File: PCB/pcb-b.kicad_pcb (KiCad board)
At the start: 2 copper layers, 116.9 x 83.4 mm, 104 parts, among them IC2 BDX34C, IC3 BDX34C, K1 RT42xxxx, Q1 D45VH10, Q10 BC337, Q11 BC337, Q12 BC327, Q13 BC337, Q14 D45VH10, Q15 D45VH10, Q16 BC337, Q17 BC337, Q18 BC327, Q19 BC327, Q2 D45VH10, Q20 BC327, Q3 BC337, Q4 BC337, Q5 BC337, Q6 BC337, Q7 BC337, Q8 BC337, Q9 BC337, U1 L7805, U2 L7805, U3 L7805, U4 ATmega16L-8P

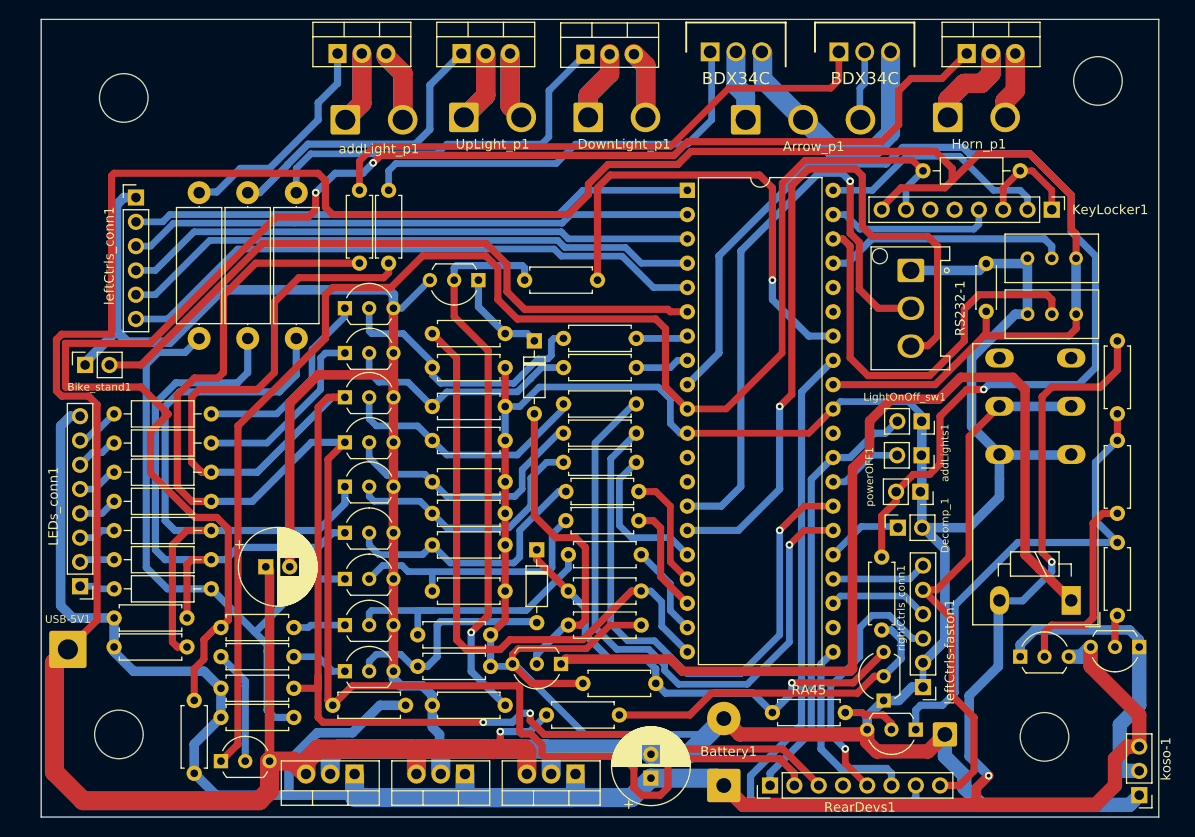
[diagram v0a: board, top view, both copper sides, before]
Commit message: fixes
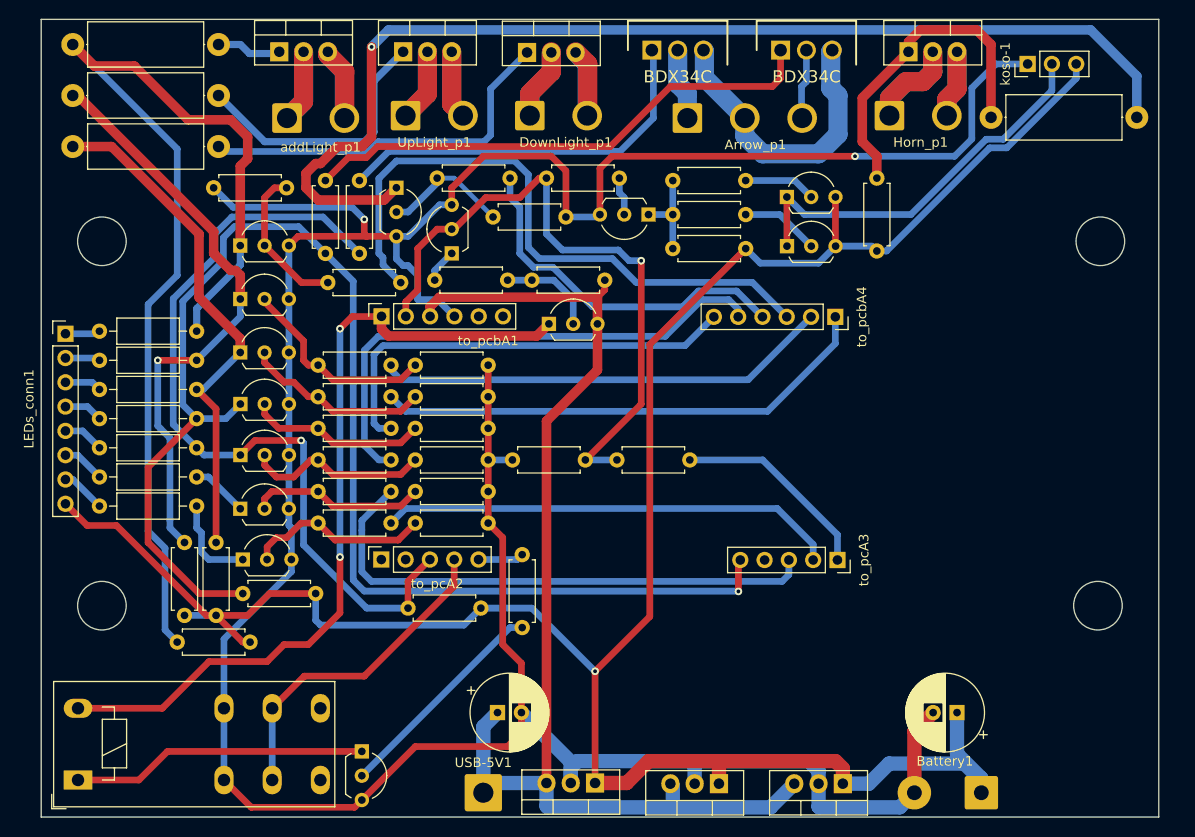
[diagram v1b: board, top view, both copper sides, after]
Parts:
- removed Bike_stand1, Decomp_1, LightOnOff_sw1, addLights1, powerOFF1: Conn_01x02, Connector_PinSocket_2.54mm:PinSocket_1x02_P2.54mm_Vertical
- removed C2: 100nF, Capacitor_THT:C_Disc_D4.3mm_W1.9mm_P5.00mm
- removed D3, D4: 2V, Diode_THT:D_DO-35_SOD27_P7.62mm_Horizontal
- removed KeyLocker1, RearDevs1: Conn_01x08, Connector_PinHeader_2.54mm:PinHeader_1x08_P2.54mm_Vertical
- removed Q19, Q20: BC327, Package_TO_SOT_THT:TO-92L_Inline_Wide
- removed R1: 1K, Resistor_THT:R_Axial_DIN0207_L6.3mm_D2.5mm_P10.16mm_Horizontal
- removed RA45: 10K, Resistor_THT:R_Axial_DIN0207_L6.3mm_D2.5mm_P7.62mm_Horizontal
- removed RA46, RA47: 3K, Resistor_THT:R_Axial_DIN0207_L6.3mm_D2.5mm_P7.62mm_Horizontal
- removed RA48, RA49: 100K, Resistor_THT:R_Axial_DIN0207_L6.3mm_D2.5mm_P7.62mm_Horizontal
- removed RS232-1: Conn_01x03, Connector_Hirose:Hirose_DF63M-3P-3.96DSA_1x03_P3.96mm_Vertical
- removed RV1, RV2: 10K, Potentiometer_THT:Potentiometer_Bourns_3296W_Vertical
- removed U4: ATmega16L-8P, Package_DIP:DIP-40_W15.24mm
- removed leftCtrls-faston1: Conn_01x01, Connector_Wire:SolderWire-0.75sqmm_1x01_D1.25mm_OD2.3mm
- removed leftCtrls_conn1, rightCtrls_conn1: Conn_01x06, Connector_PinHeader_2.54mm:PinHeader_1x06_P2.54mm_Vertical
- added to_pcA2: Conn_01x05, Connector_PinSocket_2.54mm:PinSocket_1x05_P2.54mm_Vertical, F.Cu at (135.1, 112.2)
- added to_pcA3: Conn_01x05, Connector_PinSocket_2.54mm:PinSocket_1x05_P2.54mm_Vertical, F.Cu at (182.8, 112.2)
- added to_pcbA1: Conn_01x06, Connector_PinSocket_2.54mm:PinSocket_1x06_P2.54mm_Vertical, F.Cu at (135.2, 86.7)
- added to_pcbA4: Conn_01x06, Connector_PinSocket_2.54mm:PinSocket_1x06_P2.54mm_Vertical, F.Cu at (182.6, 86.8)
- Q12: value BC327 -> BC337
- Q16, Q17: value BC337 -> BC327
- RA15: footprint Resistor_THT:R_Axial_DIN0207_L6.3mm_D2.5mm_P7.62mm_Horizontal -> Resistor_THT:R_Axial_DIN0414_L11.9mm_D4.5mm_P15.24mm_Horizontal
- RA23: value 5K -> 100K
- RA29: value 10K -> 1K
- RA31: value 100K -> 3K
- RA33: value 10K -> 3K
- RA41: value 4K -> 100K
- RA43, RA44: value 100K -> 10K
- RA7: value 1K -> 5K
- RA8: value 4K -> 10K
- moved K1 105.5 mm to (103.4, 135.2), turned to 0 degrees
- moved RA15 103.0 mm to (214.1, 65.9)
- moved RA42 89.9 mm to (187.0, 79.9)
- moved koso-1 77.3 mm to (202.7, 60.3), turned to 90 degrees
- moved RA29 59.3 mm to (140.7, 82.9), turned to 0 degrees
- moved Q12 58.3 mm to (142.5, 80.2), turned to 90 degrees
- moved Q16 57.2 mm to (152.7, 87.5), turned to 0 degrees
- moved Q18 53.6 mm to (177.5, 74.3), turned to 0 degrees
- moved RA7 52.2 mm to (141.0, 72.3), turned to 0 degrees
- moved RA30 51.2 mm to (165.6, 79.6)
- moved Q13 47.9 mm to (163.1, 76.1)
- moved RA31 46.8 mm to (173.2, 76.1), turned to 180 degrees
- moved Q9 46.0 mm to (136.7, 73.3), turned to -90 degrees
- moved USB-5V1 45.9 mm to (145.8, 136.5)
- moved RA34 44.8 mm to (125.2, 73.3), turned to 180 degrees
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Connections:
- K1 pad A2: +12V -> tempPower
- Q11 pad 1: Net-(Q11-Pad1) -> Net-(K1-PadA1)
- Q11 pad 2: Net-(D4-Pad2) -> Net-(Q11-Pad2)
- Q12 pad 1: tempPower -> Net-(Q12-Pad1)
- Q12 pad 2: Net-(Q12-Pad2) -> i_powerOFF
- Q12 pad 3: +5V -> GND
- Q13 pad 1: Net-(K1-PadA1) -> Net-(Q13-Pad1)
- Q13 pad 2: Net-(D3-Pad2) -> Net-(Q13-Pad2)
- Q16 pad 1: Net-(Q16-Pad1) -> tempPower
- Q16 pad 3: GND -> +5V
- Q17 pad 1: Net-(D3-Pad1) -> Net-(Q17-Pad1)
- Q17 pad 3: GND -> +12V
- Q18 pad 1: GND -> Net-(Q17-Pad1)
- Q18 pad 3: Net-(D4-Pad1) -> +12V
- RA23 pad 1: Net-(Q9-Pad2) -> Net-(Q16-Pad2)
- RA23 pad 2: o_horn -> +5V
- RA29 pad 1: Net-(Q18-Pad2) -> Net-(Q12-Pad1)
- RA29 pad 2: i_powerOFF -> Net-(Q16-Pad2)
- RA30 pad 1: Net-(D4-Pad2) -> Net-(Q13-Pad1)
- RA30 pad 2: GND -> +12V
- RA31 pad 1: Net-(D3-Pad2) -> Net-(Q17-Pad2)
- RA31 pad 2: GND -> Net-(Q13-Pad1)
- RA33 pad 1: Net-(Q17-Pad2) -> Net-(Q18-Pad2)
- RA33 pad 2: o_engineOFF -> Net-(Q13-Pad1)
- RA41 pad 1: Net-(D3-Pad1) -> i_powerOFF
- RA41 pad 2: o_keepAlive -> GND
- RA43 pad 1: GND -> i_powerOFF
- RA43 pad 2: Net-(Q17-Pad2) -> o_keepAlive
- RA44 pad 1: +5V -> Net-(Q11-Pad2)
- RA44 pad 2: Net-(Q18-Pad2) -> o_engineON
- RA7 pad 1: Net-(Q11-Pad1) -> Net-(Q9-Pad2)
- RA7 pad 2: Net-(Q12-Pad2) -> o_horn
- RA8 pad 1: Net-(D4-Pad1) -> i_powerOFF
- RA8 pad 2: o_keepAlive -> Net-(Q13-Pad2)
- koso-1 pad 2: Net-(Q19-Pad1) -> Net-(Q17-Pad1)
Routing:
- net +5V: track 328.6 -> 122.0 mm, vias 1 -> 0
- net GND: track 478.3 -> 332.3 mm, vias 0 -> 2
- net Net-(Q15-Pad1): track 163.5 -> 34.3 mm, vias 2 -> 0
- net Net-(Q9-Pad1): track 5.44 -> 116.9 mm, vias 0 -> 1
- net Net-(U4-Pad15): track 78.8 -> 0.00 mm, vias 1 -> 0
- net i_bykeStand: track 70.3 -> 0.00 mm
- net tempPower: track 156.0 -> 85.8 mm, vias 0 -> 2
- net Net-(K1-PadA1): track 100.7 -> 30.9 mm
- net c_rightArrow: track 153.8 -> 85.2 mm, vias 2 -> 1
- net i_neutral: track 68.3 -> 0.00 mm
- net Net-(RS232-1-Pad2): track 64.1 -> 0.00 mm, vias 1 -> 0
- net i_horn: track 62.3 -> 0.00 mm
- net i_rightArrow: track 61.0 -> 0.00 mm
- net i_upLight: track 59.6 -> 0.00 mm
- net i_leftArrow: track 59.0 -> 0.00 mm
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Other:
- outline, holes or cut-outs redrawn
